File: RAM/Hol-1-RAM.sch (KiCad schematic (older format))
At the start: 22 parts, among them P1 ADDRESS PORT, P2 DATA PORT, P3 DATA BUS, P4 Power, U1 74LS139, U10 74LS04, U11 74LS04, U12 74LS245, U2 74LS189, U3 74LS189, U4 74LS189, U5 74LS189, U6 74LS189, U7 74LS189, U8 74LS189, U9 74LS189

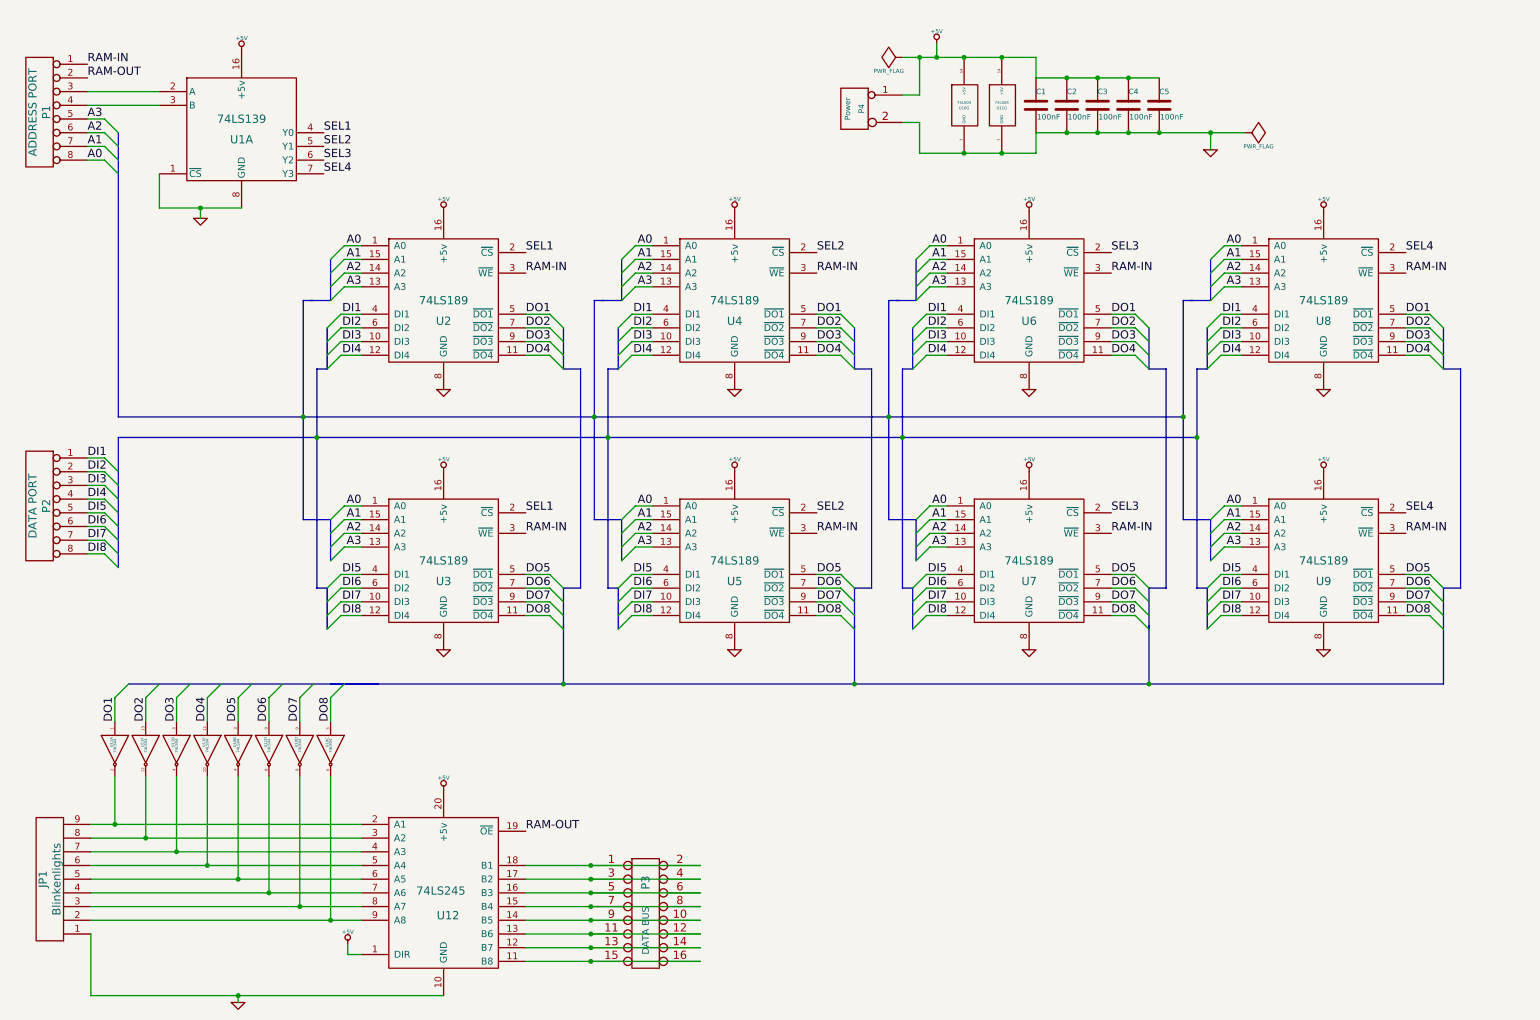
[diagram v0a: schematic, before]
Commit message: v1.1.2 comments added to schematic
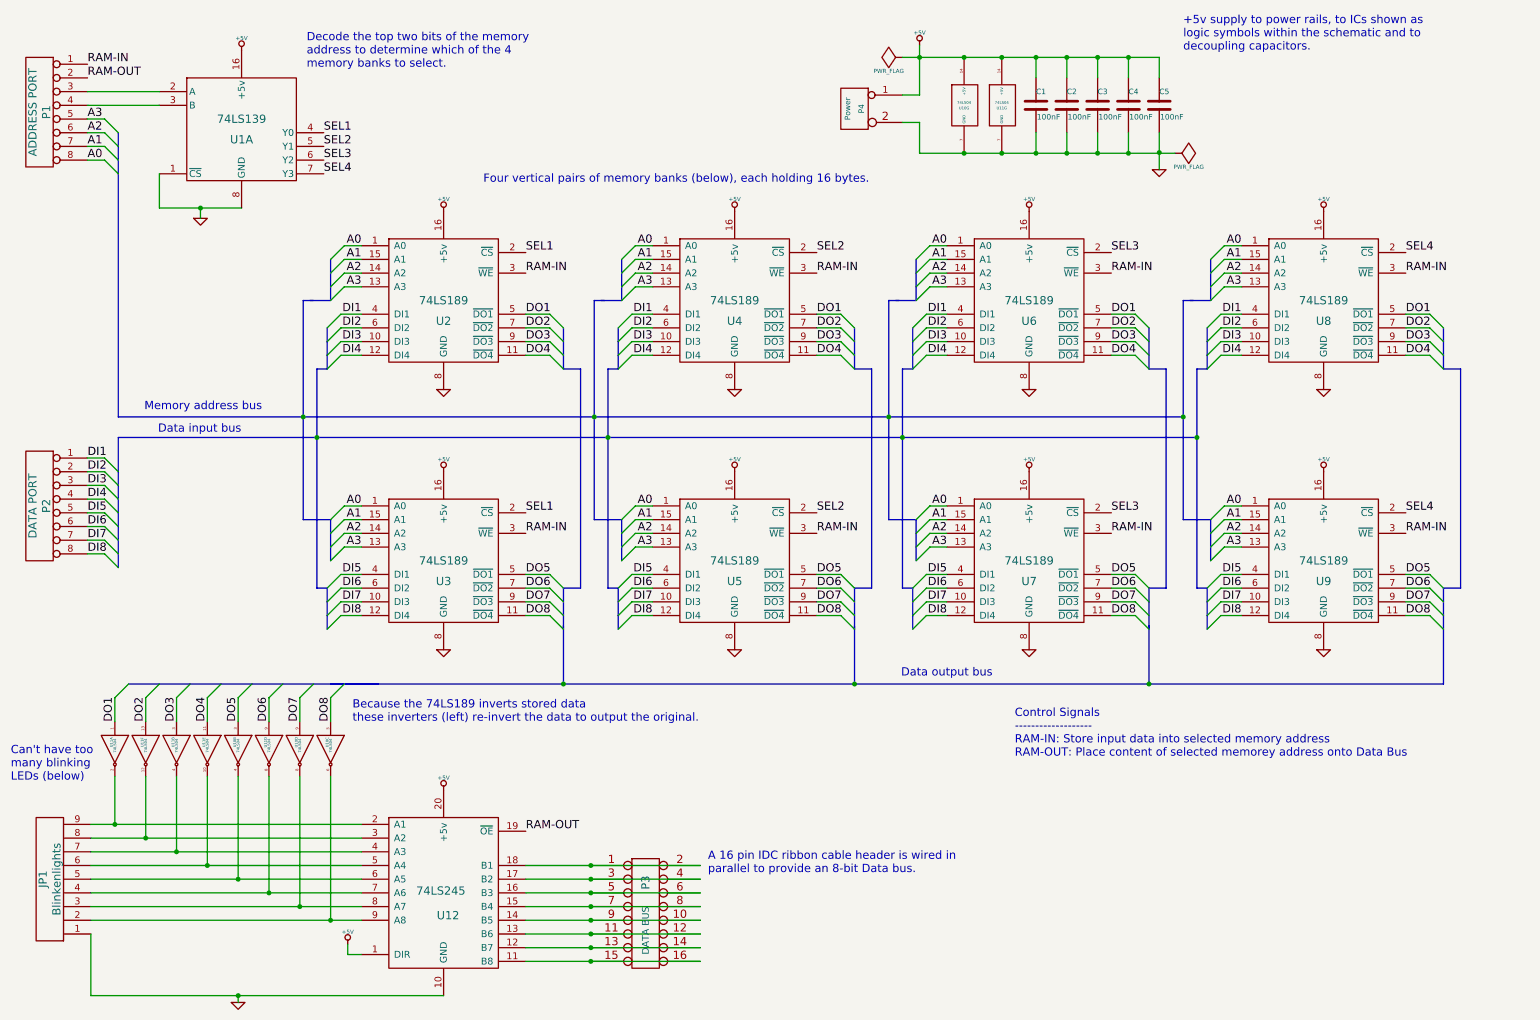
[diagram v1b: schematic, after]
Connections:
- net GND: no longer C1.2, C2.2, C3.2, C4.2, P4.2 (PM), U10.7 (GND), U11.7 (GND)
- new net: C1.2, C2.2, C3.2, C4.2, P4.2 (PM), U10.7 (GND), U11.7 (GND)
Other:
- note added: "+5v supply to power rails, to ICs shown as\nlogic symbols within the schematic and to\ndecoupling capacitors."
- note added: "A 16 pin IDC ribbon cable header is wired in\nparallel to provide an 8-bit Data bus."
- note added: "Because the 74LS189 inverts stored data\nthese inverters (left) re-invert the data to output the original."
- note added: "Can't have too\nmany blinking\nLEDs (below)"
- note added: "Control Signals\n-------------------\nRAM-IN: Store input data into selected memory address\nRAM-OUT: Place content of selected memorey address onto Data Bus"
- note added: "Data input bus"
- note added: "Data output bus"
- note added: "Decode the top two bits of the memory\naddress to determine which of the 4\nmemory banks to select."
- note added: "Four vertical pairs of memory banks (below), each holding 16 bytes."
- note added: "Memory address bus"
